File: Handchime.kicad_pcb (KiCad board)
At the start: 4 copper layers, 38.1 x 22.6 mm, 18 parts, among them J1 USB_C_Receptacle_USB2.0, J2 Pins, SW0 BOOT, SW1 Row 0, Col 0, SW2 Row 0, Col 1, U1 CH552T, U2 PRTR5V0U2X

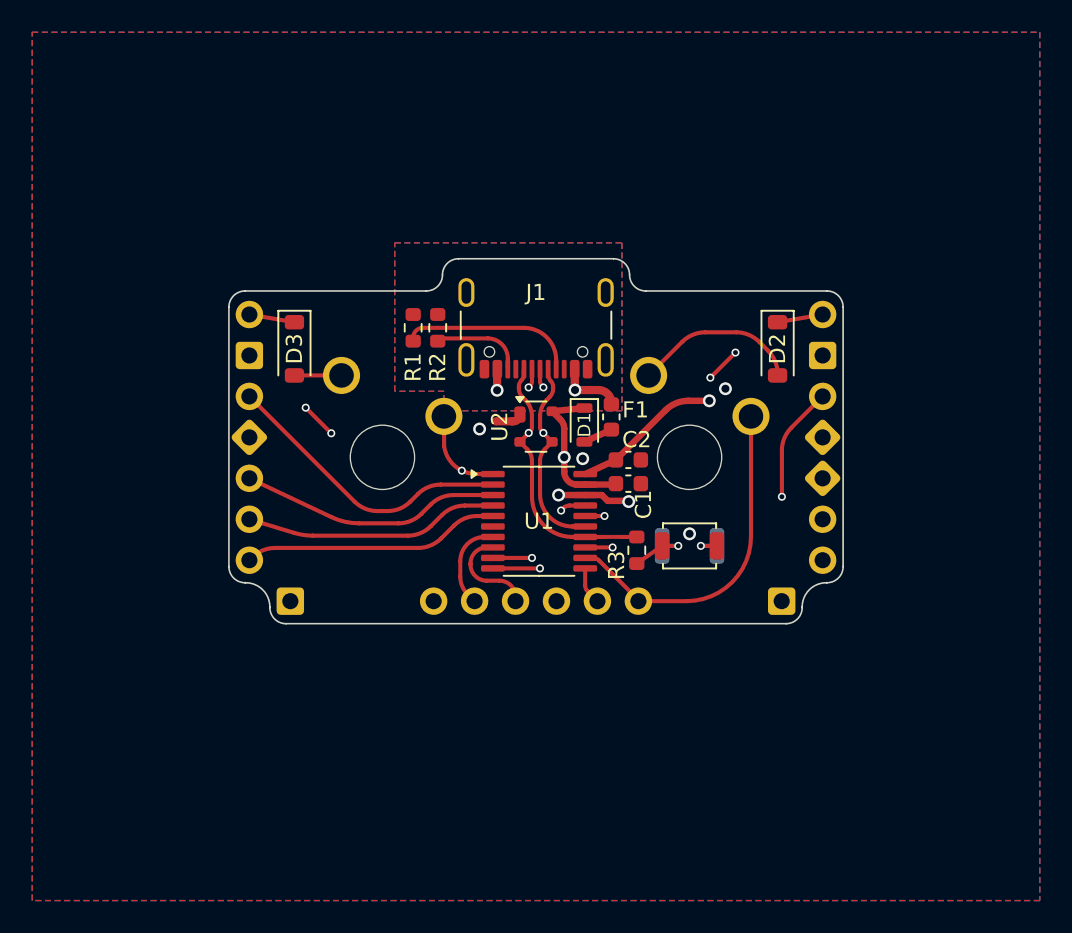
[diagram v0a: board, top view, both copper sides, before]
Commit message: Update PCB with STH32 version draft
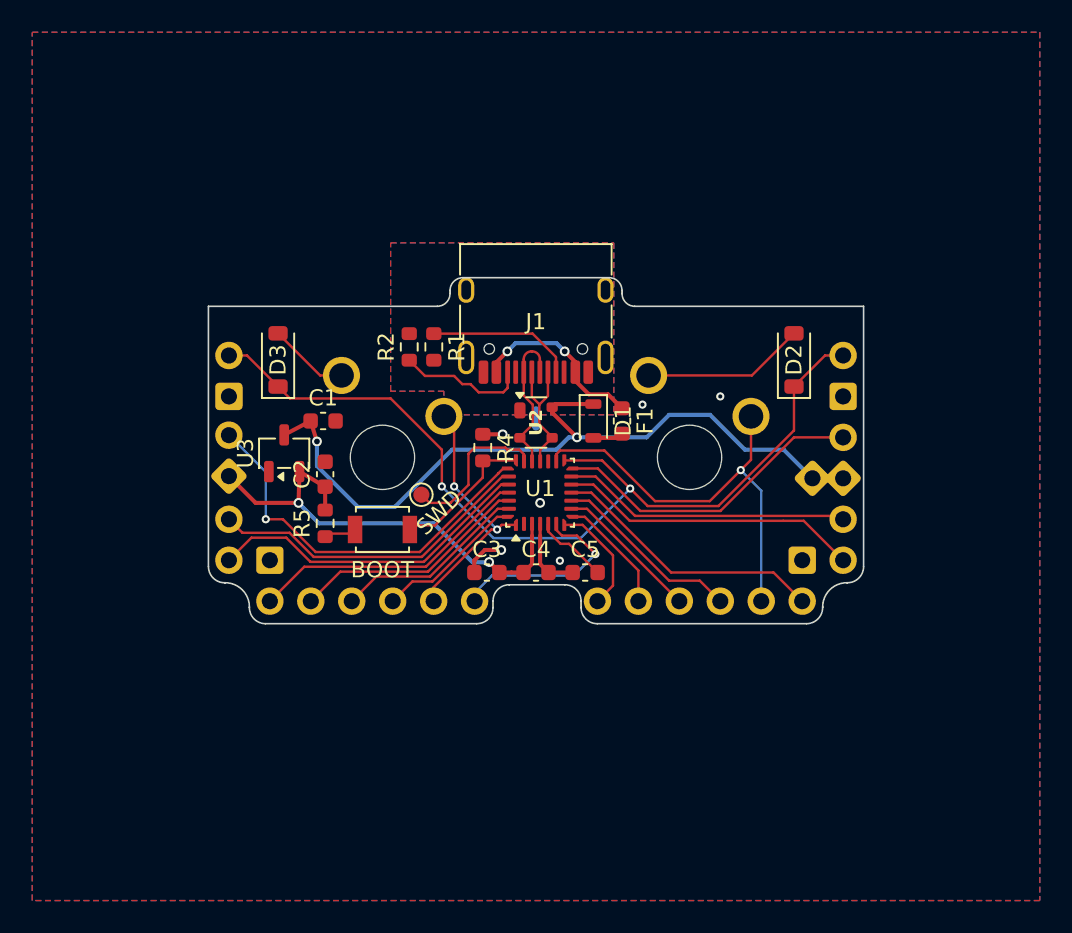
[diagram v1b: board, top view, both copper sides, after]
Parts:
- removed NT2: NetTie_2, Project Library:NetTie-2_SMD_Pad0.254mm
- removed R3: 5.1k, Resistor_SMD:R_0603_1608Metric
- added C3: 4.7µF, Capacitor_SMD:C_0603_1608Metric, F.Cu at (155.7, 57.1)
- added C4: 100nF, Capacitor_SMD:C_0603_1608Metric, F.Cu at (158.8, 57.1)
- added C5: 100nF, Capacitor_SMD:C_0603_1608Metric, F.Cu at (161.8, 57.1)
- added J3: SWD, TestPoint:TestPoint_Pad_D1.0mm, F.Cu at (151.6, 52.3)
- added R4: 10kΩ, Resistor_SMD:R_0603_1608Metric, F.Cu at (155.4, 49.4)
- added R5: 330Ω, Resistor_SMD:R_0603_1608Metric, F.Cu at (145.7, 54.1)
- added U3: XC6206P332MR-G, Package_TO_SOT_SMD:SOT-23-3, F.Cu at (143.1, 49.8)
- C1, C2: value 100nF -> 1µF
- D1: footprint Project Library:D_SOD-323 -> BGK_Kicad:D_SOD-323
- J1: value USB_C_Receptacle_USB2.0 -> USB_C_Receptacle_USB2.0_16P; footprint Connector_USB:USB_C_Receptacle_GCT_USB4105-xx-A_16P_TopMnt_Horizontal -> Connector_USB:USB_C_Receptacle_HRO_TYPE-C-31-M-12
- NT1: moved to B.Cu
- SW0: footprint Project Library:SW_SPST_B3U-1000P -> Button_Switch_SMD:SW_SPST_B3U-1000P
- U1: value CH552T -> STM32C071GBUx; footprint Package_SO:TSSOP-20_4.4x6.5mm_P0.65mm -> Package_DFN_QFN:QFN-28_4x4mm_P0.5mm
- moved C1 19.3 mm to (145.5, 47.8)
- moved SW0 19.1 mm to (149.2, 54.5), turned to 180 degrees
- moved C2 18.8 mm to (145.7, 51.1), turned to 90 degrees
- moved R2 2.13 mm to (150.9, 43.2)
- moved NT1 2.01 mm to (158.8, 47.6), turned to -90 degrees
- moved U1 1.78 mm to (159.0, 52.2), turned to 90 degrees
- moved R1 1.74 mm to (152.4, 43.2), turned to -90 degrees
- moved D2 1.23 mm to (174.8, 44.0), turned to 90 degrees
- moved D3 1.23 mm to (142.7, 44.0), turned to 90 degrees
- moved F1 0.71 mm to (164.1, 47.8)
- moved D1 0.61 mm to (162.3, 47.8)
- moved U2 0.25 mm to (158.8, 47.8)
- moved J1 0.18 mm to (158.7, 40.7)
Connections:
- J1 pad A1: GNDPWR -> ISLAND
- J1 pad A12: GNDPWR -> ISLAND
- J1 pad B1: GNDPWR -> ISLAND
- J1 pad B12: GNDPWR -> ISLAND
- J2 pad 1: R0 -> VCC
- J2 pad 10: P10 -> PB7
- J2 pad 11: P11 -> PB8
- J2 pad 12: P13 -> C1
- J2 pad 13: P33 -> PA0
- J2 pad 14: C0 -> PA1
- J2 pad 15: GND -> PA2
- J2 pad 16: TX -> PA3
- J2 pad 17: RX -> PA4
- J2 pad 18: +3V3 -> C0
- J2 pad 19: VCC -> PA5
- J2 pad 2: GND -> +3V3
- J2 pad 20: P35 -> PA6
- J2 pad 21: GND -> PA7
- J2 pad 22: R0 -> PB0
- J2 pad 3: P14 -> GND
- J2 pad 4: VCC -> R0
- J2 pad 5: P15 -> PA15
- J2 pad 6: P16 -> PB3
- J2 pad 7: P17 -> PB4
- J2 pad 8: GND -> PB5
- J2 pad 9: C1 -> PB6
- NT1 pad 1: GNDPWR -> ISLAND
- R1 pad 2: GNDPWR -> ISLAND
- R2 pad 2: GNDPWR -> ISLAND
- SW0 pad 1: Net-(R3-Pad2) -> BOOT0/SWCLK
- SW0 pad 2: +3V3 -> Net-(R5-Pad1)
- U1 pad 10: TX -> PA4
- U1 pad 11: P33 -> PA5
- U1 pad 12: C0 -> PA6
- U1 pad 13: P35 -> PA7
- U1 pad 14: USB+ -> PB0
- U1 pad 15: USB- -> R0
- U1 pad 16: P13 -> C0
- U1 pad 17: R0 -> unconnected-(U1-PC6-Pad17)
- U1 pad 18: GND -> USB-
- U1 pad 19: VCC -> USB+
- U1 pad 2: P14 -> unconnected-(U1-PC15-Pad2)
- U1 pad 20: +3V3 -> SWDIO
- U1 pad 3: P15 -> +3V3
- U1 pad 4: P16 -> GND
- U1 pad 5: P17 -> NRST
- U1 pad 6: RST -> PA0
- U1 pad 7: P10 -> PA1
- U1 pad 8: P11 -> PA2
- U1 pad 9: RX -> PA3
- U2 pad 1: GNDPWR -> ISLAND
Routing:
- net PA15: track 0.00 -> 24.2 mm, vias 0 -> 1
- net RX: track 21.4 -> 0.00 mm, vias 1 -> 0
- net P35: track 21.1 -> 0.00 mm, vias 2 -> 0
- net TX: track 20.9 -> 0.00 mm, vias 1 -> 0
- net PB4: track 0.00 -> 20.6 mm
- net PB3: track 0.00 -> 20.4 mm
- net PB0: track 0.00 -> 19.8 mm
- net PA6: track 0.00 -> 18.8 mm
- net P14: track 18.4 -> 0.00 mm
- net PA7: track 0.00 -> 18.0 mm
- net PB5: track 0.00 -> 17.6 mm
- net PA5: track 0.00 -> 17.1 mm
- net P15: track 16.2 -> 0.00 mm
- net P17: track 16.0 -> 0.00 mm
- net P16: track 15.8 -> 0.00 mm
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- added copper zone on In2.Cu, net GND
- added copper zone on B.Cu, net ISLAND
- added copper zone on F.Cu, net ISLAND
- added copper zone on In1.Cu, net ISLAND
- added copper zone on In2.Cu, net ISLAND
- removed copper zone on B.Cu, net GNDPWR
- removed copper zone on F.Cu, net GNDPWR
- removed copper zone on In1.Cu, net GNDPWR
- removed copper zone on In2.Cu, net GNDPWR
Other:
- board size 38.1 x 22.6 mm -> 40.6 x 21.5 mm
- board text added: "USB Port Y should be 42.164mm"
- board text added: "v2.0 • bgkendall"
- board text removed: "v1.0 • bgkendall"

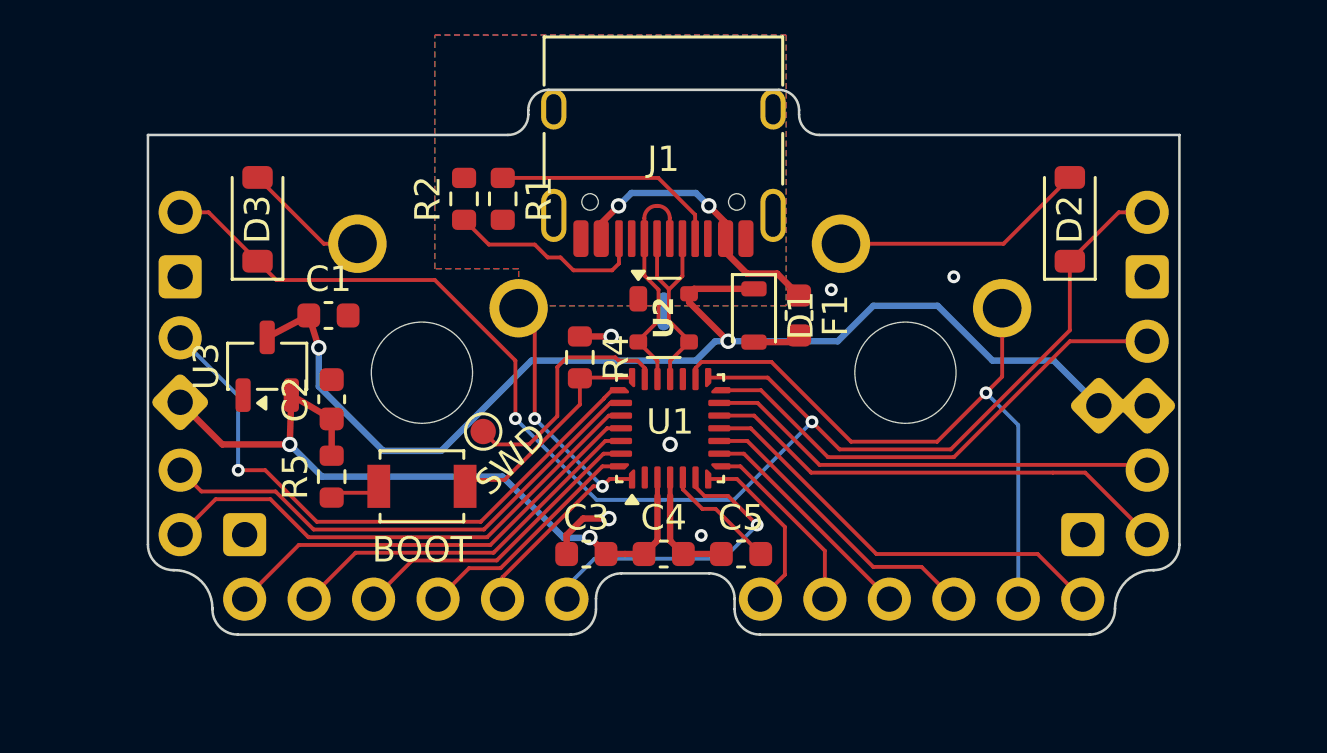
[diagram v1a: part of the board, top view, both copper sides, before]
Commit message: Various tweaks and improvements
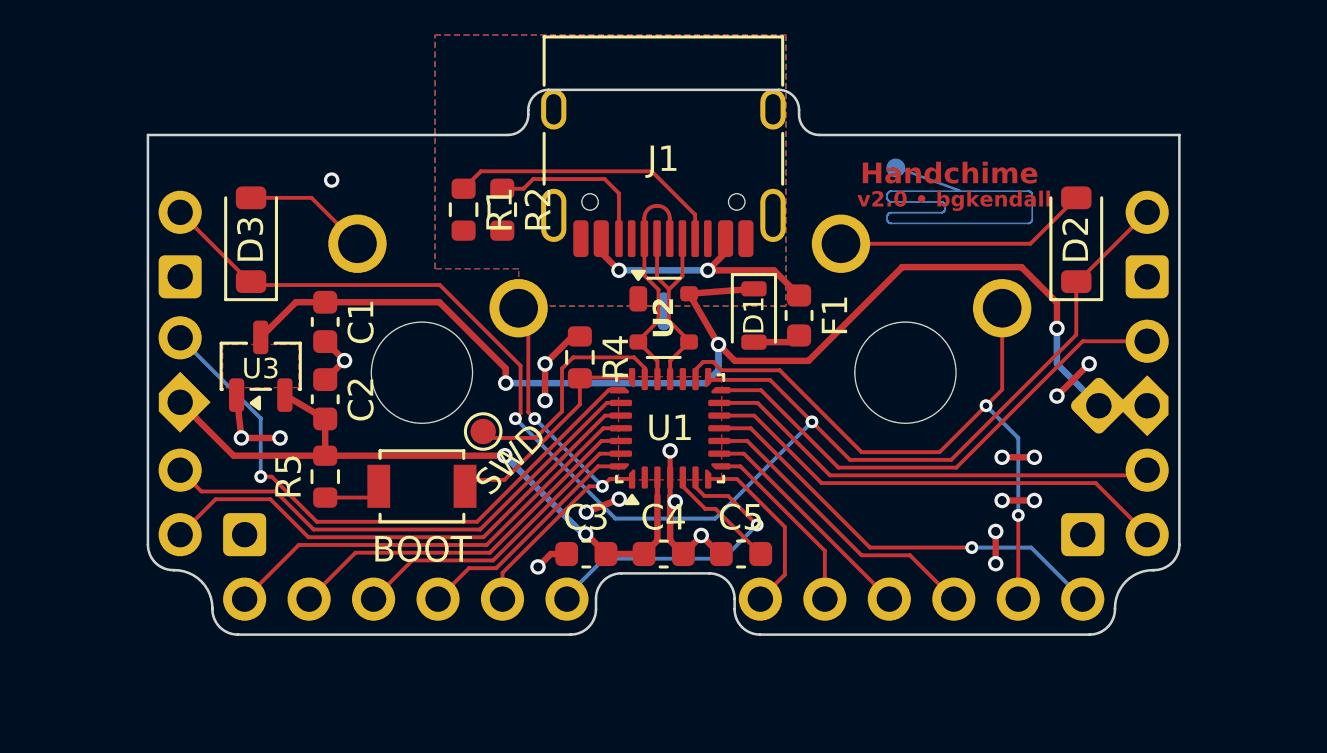
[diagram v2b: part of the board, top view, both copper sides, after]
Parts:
- moved R1 1.60 mm to (150.9, 43.6)
- moved R2 1.56 mm to (152.4, 43.6), turned to -90 degrees
- moved D2 0.84 mm to (175.0, 44.8)
- moved D3 0.84 mm to (142.5, 44.8)
- moved C1 0.28 mm to (145.4, 48.0), turned to -90 degrees
- moved C2 0.25 mm to (145.4, 51.1)
- moved R5 0.25 mm to (145.4, 54.1)
- moved U3 0.25 mm to (142.9, 49.8)
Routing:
- net GND: track 8.65 -> 23.6 mm, vias 6 -> 20
- net +3V3: track 29.2 -> 27.3 mm
- net Net-(J1-CC1): track 9.12 -> 11.1 mm
- net Net-(J1-CC2): track 8.02 -> 6.77 mm
- net VCC: track 45.6 -> 46.8 mm, vias 2 -> 3
- net VBUS: track 11.3 -> 10.4 mm
- net R0: track 56.1 -> 56.9 mm
- net PA15: track 24.2 -> 23.5 mm
- net C0: track 26.3 -> 26.4 mm, vias 1 -> 2
- net PA5: vias 0 -> 1
